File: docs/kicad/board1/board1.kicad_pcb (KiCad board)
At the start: 2 copper layers, 98 x 96 mm, 42 parts, among them J1 12V_IN, J2 5V_JUMP, J3 MINI_BOX, J4 MECH_THERM, J5 EXT_LED, J6 LCD, J7 TEMP1, J8 TEMP2, J9 12V_TEST, M1 BUCK01, M2 SD_TYP0, Q1 BC547, SW1 ON/OFF, SW2 BUTTON1, SW3 BUTTON2, SW4 BUTTON3, U1 ESP32_DEV_0

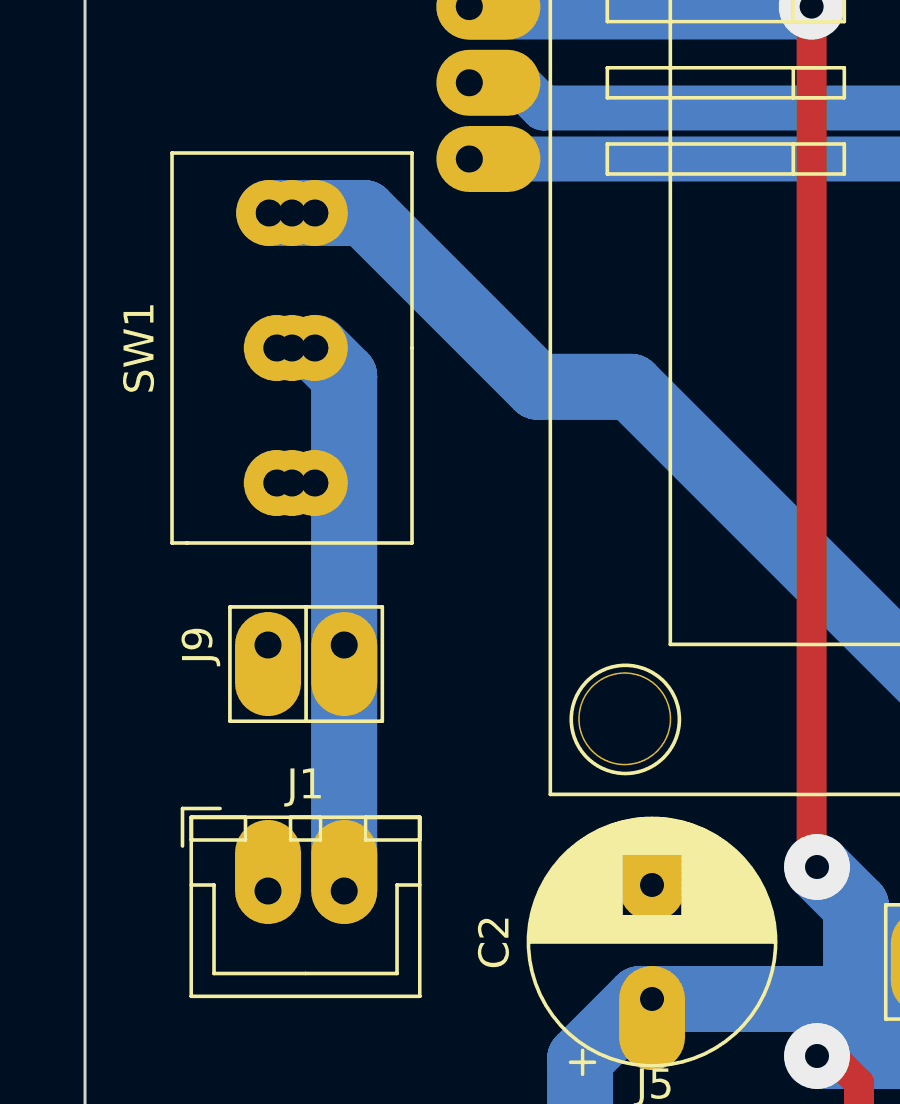
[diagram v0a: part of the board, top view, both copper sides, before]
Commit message: minor changes before more testing ArduinoIDE2.3.3 and Esp32Core3.0.4 on LENOVO-T490-2
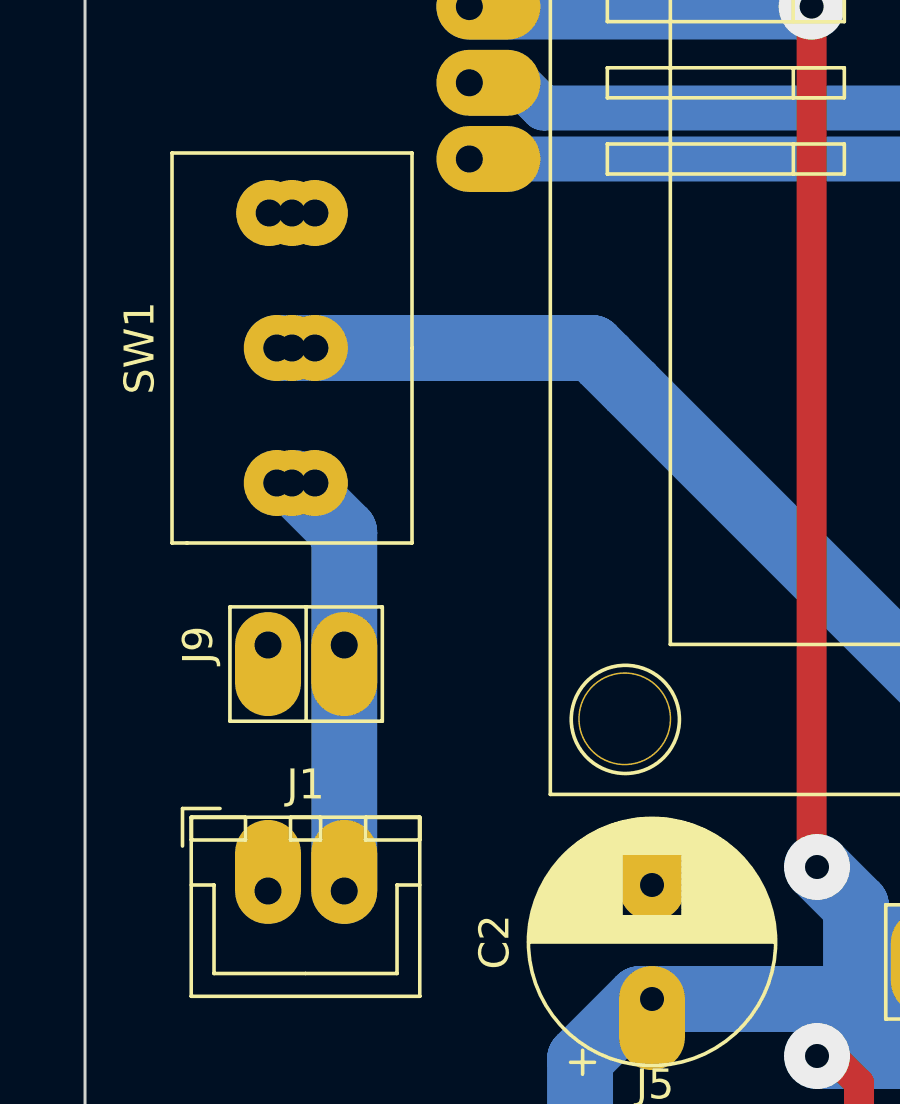
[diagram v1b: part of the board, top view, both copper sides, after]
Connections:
- J9 pad 2: Net-(J1-Pad2) -> Net-(J9-Pad2)
- SW1 pad 1: Net-(M1-Pad4) -> Net-(SW1-Pad1)
- SW1 pad 2: Net-(J1-Pad2) -> Net-(M1-Pad4)
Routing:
- net Net-(J1-Pad2): track 18.5 -> 14.3 mm
- net Net-(M1-Pad4): track 30.6 -> 28.5 mm
